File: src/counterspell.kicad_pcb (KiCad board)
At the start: 2 copper layers, 51 x 96.3 mm, 10 parts, among them SW1 SW_Push

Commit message: Update counterspell.kicad_pcb
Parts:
- added G***: LOGO, LOGO, B.Cu at (252.1, 81.3)
- added G***: LOGO, LOGO, B.Cu at (242.6, 75.6)

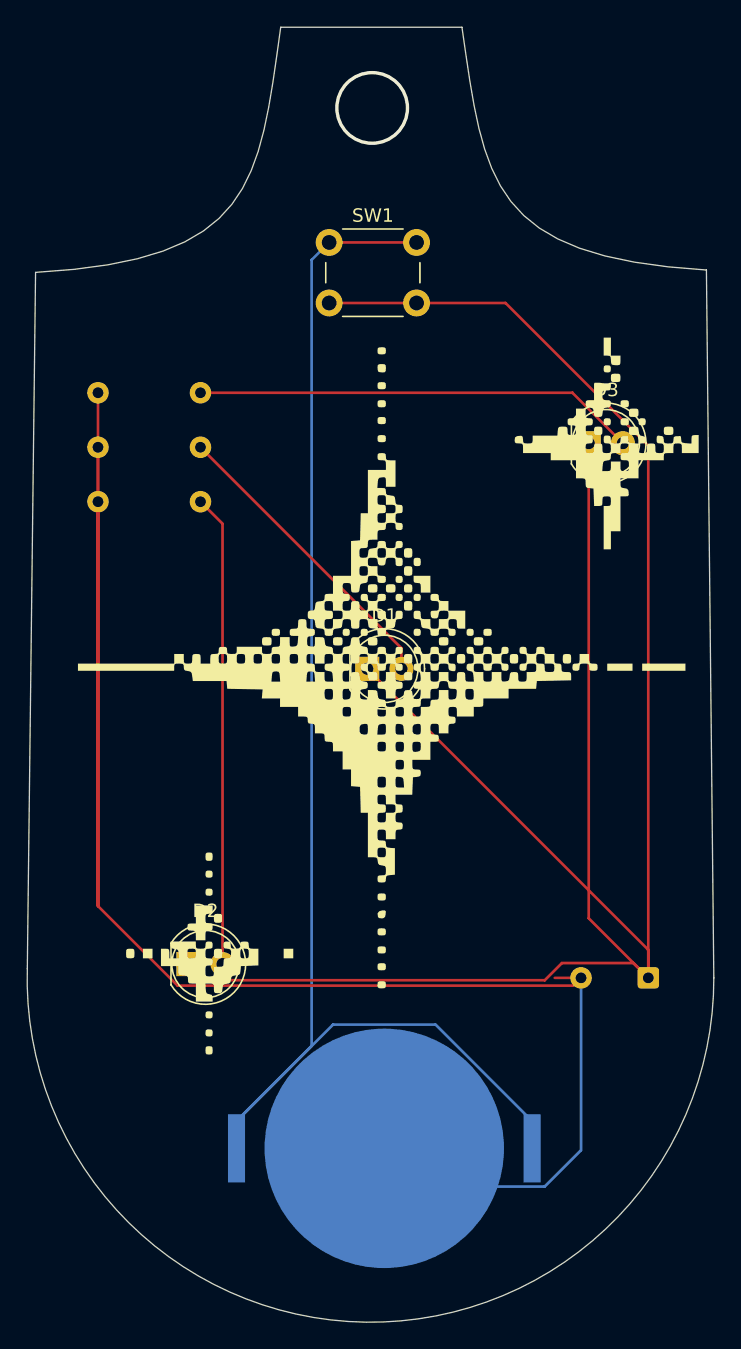
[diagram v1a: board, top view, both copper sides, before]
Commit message: important
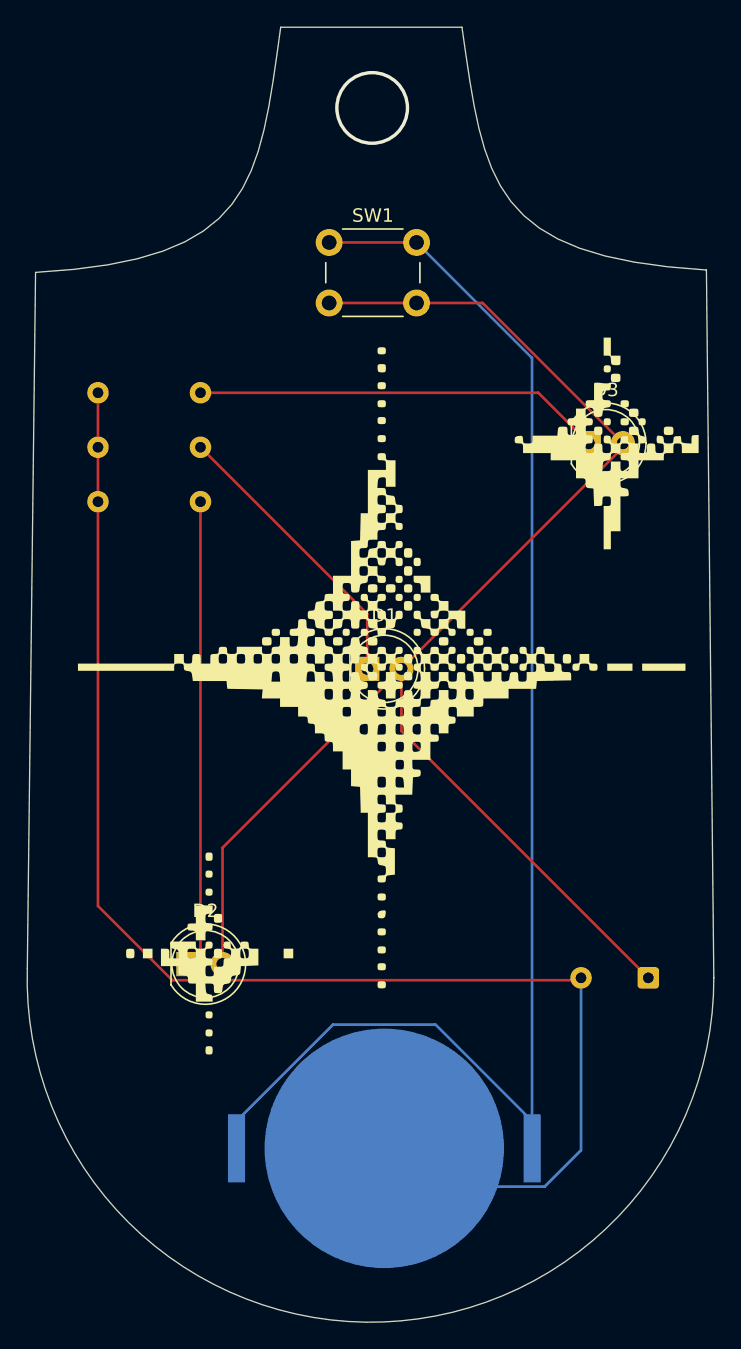
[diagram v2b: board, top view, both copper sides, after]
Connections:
- C1 pad 1: Net-(D1-K) -> Net-(D1-A)
- D2 pad 1: Net-(D1-K) -> Net-(D2-K)
- D2 pad 2: Net-(D2-A) -> Net-(D1-A)
- D3 pad 1: Net-(D1-K) -> Net-(D3-K)
- D3 pad 2: Net-(D3-A) -> Net-(D1-A)
- R1 pad 1: Net-(D3-A) -> Net-(D3-K)
- R2 pad 1: Net-(D1-A) -> Net-(D1-K)
- R3 pad 1: Net-(D2-A) -> Net-(D2-K)
- SW1 pad 2: Net-(D1-K) -> Net-(D1-A)
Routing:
- net Net-(D1-K): track 176.6 -> 21.6 mm
- net Net-(D1-A): track 22.7 -> 107.8 mm
- net Net-(BT1--): track 172.6 -> 106.2 mm
- net Net-(D2-A): track 35.1 -> 0.00 mm
- net Net-(D2-K): track 0.00 -> 34.7 mm
- net Net-(D3-A): track 33.0 -> 0.00 mm
- net Net-(D3-K): track 0.00 -> 30.4 mm
- net Net-(BT1-+): track 106.6 -> 105.3 mm
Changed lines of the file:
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@@
 	(net 3 "Net-(D1-K)")
 	(net 4 "Net-(D1-A)")
-	(net 5 "Net-(D2-A)")
-	(net 6 "Net-(D3-A)")
+	(net 5 "Net-(D2-K)")
+	(net 6 "Net-(D3-K)")
 	(footprint "LED_THT:LED_D5.0mm"
 		(layer "F.Cu")
@@
 			(layers "*.Cu" "*.Mask")
 			(remove_unused_layers no)
-			(net 3 "Net-(D1-K)")
+			(net 6 "Net-(D3-K)")
 			(pinfunction "K")
 			(pintype "passive")
@@
 			(layers "*.Cu" "*.Mask")
 			(remove_unused_layers no)
-			(net 6 "Net-(D3-A)")
+			(net 4 "Net-(D1-A)")
 			(pinfunction "A")
 			(pintype "passive")
@@
 			(layers "*.Cu" "*.Mask")
 			(remove_unused_layers no)
-			(net 3 "Net-(D1-K)")
+			(net 5 "Net-(D2-K)")
 			(pinfunction "K")
 			(pintype "passive")
@@
 			(layers "*.Cu" "*.Mask")
 			(remove_unused_layers no)
-			(net 5 "Net-(D2-A)")
+			(net 4 "Net-(D1-A)")
 			(pinfunction "A")
 			(pintype "passive")
@@
 			(layers "*.Cu" "*.Mask")
 			(remove_unused_layers no)
-			(net 3 "Net-(D1-K)")
+			(net 4 "Net-(D1-A)")
 			(pinfunction "2")
 			(pintype "passive")
@@
 			(layers "*.Cu" "*.Mask")
 			(remove_unused_layers no)
-			(net 3 "Net-(D1-K)")
+			(net 4 "Net-(D1-A)")
 			(pinfunction "2")
 			(pintype "passive")
@@
 			(remove_unused_layers no)
 			(roundrect_rratio 0.15625)
-			(net 3 "Net-(D1-K)")
+			(net 4 "Net-(D1-A)")
 			(pintype "passive")
 		)
@@
 			(layers "*.Cu" "*.Mask")
 			(remove_unused_layers no)
-			(net 4 "Net-(D1-A)")
+			(net 3 "Net-(D1-K)")
 			(pintype "passive")
 		)
@@
 			(layers "*.Cu" "*.Mask")
 			(remove_unused_layers no)
-			(net 5 "Net-(D2-A)")
+			(net 5 "Net-(D2-K)")
 			(pintype "passive")
 		)
@@
 			(layers "*.Cu" "*.Mask")
 			(remove_unused_layers no)
-			(net 6 "Net-(D3-A)")
+			(net 6 "Net-(D3-K)")
 			(pintype "passive")
 		)
@@
 	)
 	(segment
-		(start 248.650651 96.627)
-		(end 249.227651 96.05)
-		(width 0.2)
-		(layer "F.Cu")
-		(net 1)
-	)
-	(segment
 		(start 213.315 90.707)
-		(end 219.235 96.627)
+		(end 218.834 96.226)
 		(width 0.2)
 		(layer "F.Cu")
@@
 	)
 	(segment
-		(start 213.315 52.55)
-		(end 213.315 90.707)
+		(start 249.051651 96.226)
+		(end 249.227651 96.05)
 		(width 0.2)
 		(layer "F.Cu")
@@
 	)
 	(segment
-		(start 219.235 96.627)
-		(end 248.650651 96.627)
+		(start 218.834 96.226)
+		(end 249.051651 96.226)
 		(width 0.2)
 		(layer "F.Cu")
@@
 	)
 	(segment
-		(start 247.275 96.05)
-		(end 249.227651 96.05)
+		(start 213.315 52.55)
+		(end 213.315 56.6)
 		(width 0.2)
 		(layer "F.Cu")
@@
 	(segment
 		(start 213.315 56.6)
-		(end 213.315 90.707)
+		(end 213.315 60.65)
 		(width 0.2)
 		(layer "F.Cu")
@@
 	)
 	(segment
-		(start 249.227651 108.859349)
-		(end 249.227651 96.05)
+		(start 237.441 111.566)
+		(end 246.521 111.566)
 		(width 0.2)
 		(layer "B.Cu")
@@
 	)
 	(segment
-		(start 237.441 111.566)
-		(end 246.521 111.566)
+		(start 249.227651 108.859349)
+		(end 249.227651 96.05)
 		(width 0.2)
 		(layer "B.Cu")
@@
 	)
 	(segment
-		(start 229.199 42.676)
-		(end 230.5 41.375)
-		(width 0.2)
-		(layer "B.Cu")
-		(net 2)
-	)
-	(segment
-		(start 223.615 108.725)
-		(end 223.615 106.697821)
-		(width 0.2)
-		(layer "B.Cu")
-		(net 2)
-	)
-	(segment
-		(start 229.199 101.113821)
-		(end 229.199 42.676)
+		(start 245.585 49.96)
+		(end 237 41.375)
 		(width 0.2)
 		(layer "B.Cu")
@@
 	)
 	(segment
-		(start 223.615 106.697821)
-		(end 229.199 101.113821)
+		(start 245.585 108.725)
+		(end 245.585 49.96)
 		(width 0.2)
 		(layer "B.Cu")
@@
 	)
 	(segment
-		(start 245.585 106.697821)
-		(end 245.585 108.725)
-		(width 0.2)
-		(layer "B.Cu")
-		(net 2)
-	)
-	(segment
-		(start 237 45.875)
-		(end 243.613471 45.875)
-		(width 0.2)
-		(layer "F.Cu")
-		(net 3)
-	)
-	(segment
-		(start 220.035 95.025)
-		(end 221.236 96.226)
-		(width 0.2)
-		(layer "F.Cu")
-		(net 3)
-	)
-	(segment
-		(start 247.8089 94.949)
-		(end 253.126651 94.949)
-		(width 0.2)
-		(layer "F.Cu")
-		(net 3)
-	)
-	(segment
-		(start 243.613471 45.875)
-		(end 254.227651 56.48918)
-		(width 0.2)
-		(layer "F.Cu")
-		(net 3)
-	)
-	(segment
-		(start 230.5 45.875)
-		(end 237 45.875)
+		(start 220.935 56.6)
+		(end 233.335 69)
 		(width 0.2)
 		(layer "F.Cu")
@@
 	)
 	(segment
-		(start 254.227651 93.967651)
+		(start 233.335 69)
 		(end 233.335 73.075)
 		(width 0.2)
@@
 	)
 	(segment
-		(start 249.8 56.3)
-		(end 249.8 91.622349)
+		(start 252.34 56.61)
+		(end 252.34 56.3)
 		(width 0.2)
 		(layer "F.Cu")
-		(net 3)
+		(net 4)
 	)
 	(segment
-		(start 221.236 96.226)
-		(end 246.5319 96.226)
+		(start 222.575 86.375)
+		(end 235.875 73.075)
 		(width 0.2)
 		(layer "F.Cu")
-		(net 3)
+		(net 4)
 	)
 	(segment
-		(start 249.8 91.622349)
-		(end 254.227651 96.05)
+		(start 235.875 73.075)
+		(end 252.34 56.61)
 		(width 0.2)
 		(layer "F.Cu")
-		(net 3)
+		(net 4)
 	)
 	(segment
-		(start 253.126651 94.949)
-		(end 254.227651 96.05)
+		(start 241.915 45.875)
+		(end 252.34 56.3)
 		(width 0.2)
 		(layer "F.Cu")
-		(net 3)
+		(net 4)
 	)
 	(segment
-		(start 254.227651 96.05)
-		(end 254.227651 93.967651)
+		(start 237 45.875)
+		(end 241.915 45.875)
 		(width 0.2)
 		(layer "F.Cu")
-		(net 3)
+		(net 4)
 	)
 	(segment
-		(start 246.5319 96.226)
-		(end 247.8089 94.949)
+		(start 235.875 73.075)
+		(end 235.875 77.697349)
 		(width 0.2)
 		(layer "F.Cu")
-		(net 3)
+		(net 4)
 	)
 	(segment
-		(start 254.227651 56.48918)
+		(start 235.875 77.697349)
 		(end 254.227651 96.05)
 		(width 0.2)
 		(layer "F.Cu")
-		(net 3)
+		(net 4)
 	)
 	(segment
-		(start 235.875 73.075)
-		(end 235.875 71.54)
+		(start 222.575 95.025)
+		(end 222.575 86.375)
 		(width 0.2)
 		(layer "F.Cu")
@@
 	)
 	(segment
-		(start 235.875 71.54)
-		(end 220.935 56.6)
+		(start 230.5 45.875)
+		(end 237 45.875)
 		(width 0.2)
 		(layer "F.Cu")
@@
 	)
 	(segment
-		(start 222.575 95.025)
-		(end 222.575 62.29)
+		(start 220.935 60.65)
+		(end 220.935 94.125)
 		(width 0.2)
 		(layer "F.Cu")
@@
 	)
 	(segment
-		(start 222.575 62.29)
-		(end 220.935 60.65)
+		(start 220.935 94.125)
+		(end 220.035 95.025)
 		(width 0.2)
 		(layer "F.Cu")
@@
 	)
 	(segment
-		(start 248.59 52.55)
-		(end 220.935 52.55)
+		(start 220.935 52.55)
+		(end 246.05 52.55)
 		(width 0.2)
 		(layer "F.Cu")
@@
 	)
 	(segment
-		(start 252.34 56.3)
-		(end 248.59 52.55)
+		(start 246.05 52.55)
+		(end 249.8 56.3)
 		(width 0.2)
 		(layer "F.Cu")

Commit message: important stuff
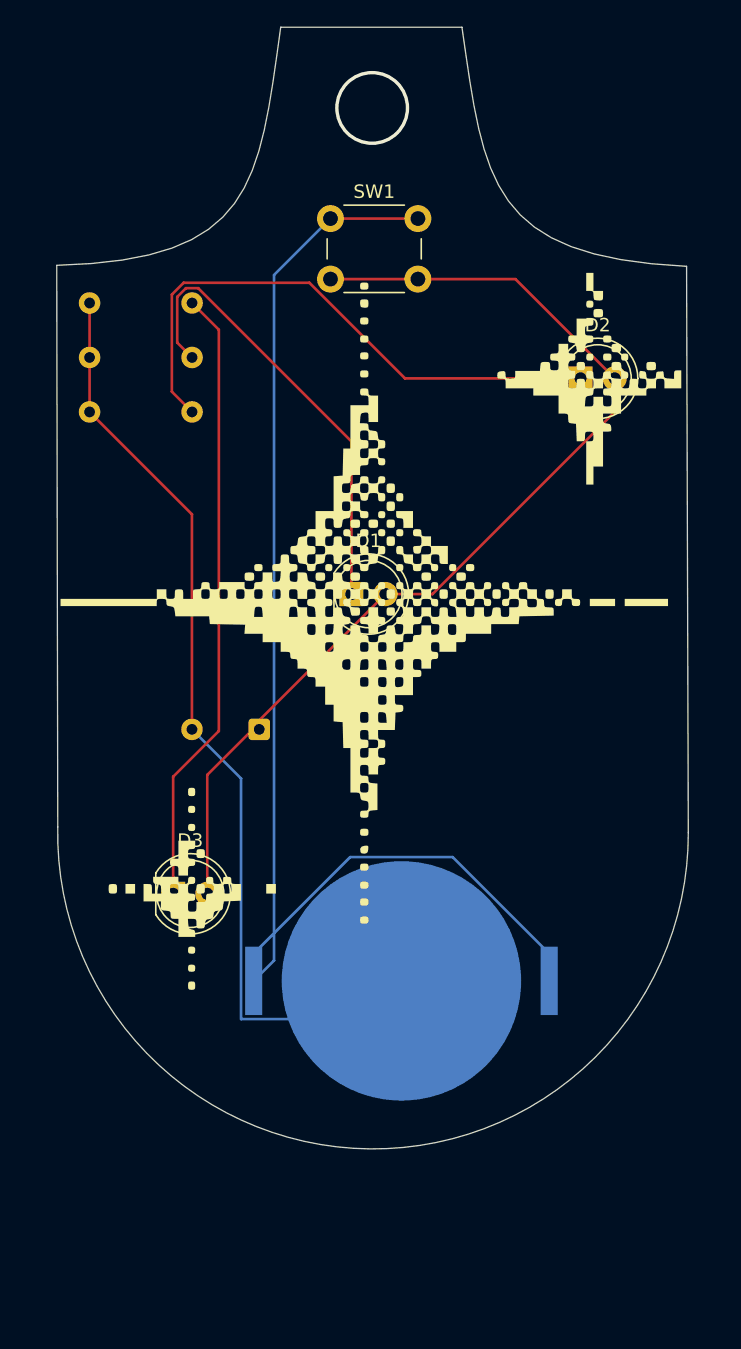
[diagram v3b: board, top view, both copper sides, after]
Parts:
- moved D2 52.4 mm to (249.2, 51.5)
- moved D3 45.6 mm to (218.9, 89.8)
- moved C1 34.3 mm to (225.3, 77.6)
- moved BT1 12.5 mm to (235.9, 96.3)
- moved R2 6.70 mm to (220.3, 49.9)
- moved R1 6.70 mm to (220.3, 45.9)
- moved R3 6.70 mm to (220.3, 54.0)
- moved D1 5.68 mm to (232.2, 67.5)
- moved G*** 4.98 mm to (250.8, 76.5)
- moved G*** 4.98 mm to (241.3, 70.8)
- moved G*** 4.98 mm to (233.6, 70.3)
- moved SW1 1.78 mm to (230.6, 39.6)
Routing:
- net Net-(BT1--): track 106.2 -> 71.0 mm
- net Net-(D1-A): track 107.8 -> 77.4 mm
- net Net-(D3-K): track 30.4 -> 46.2 mm
- net Net-(D1-K): track 21.6 -> 34.2 mm
- net Net-(D2-K): track 34.7 -> 43.0 mm
- net Net-(BT1-+): track 105.3 -> 97.5 mm
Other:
- board size 51 x 96.3 mm -> 47 x 83.4 mm
